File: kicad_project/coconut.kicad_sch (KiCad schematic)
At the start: 77 parts

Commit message: change the layout
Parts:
- K_32: footprint MX_Only:MXOnly-1U-NoLED -> MX_Only:MXOnly-1.25U-NoLED
- K_34: footprint MX_Only:MXOnly-1.5U-NoLED -> MX_Only:MXOnly-1.25U-NoLED
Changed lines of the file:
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@@
       (effects (font (size 1.524 1.524)) hide)
     )
-    (property "Footprint" "MX_Only:MXOnly-1U-NoLED" (id 2) (at 60.96 101.6 0)
+    (property "Footprint" "MX_Only:MXOnly-1.25U-NoLED" (id 2) (at 60.96 101.6 0)
       (effects (font (size 1.524 1.524)) hide)
     )
@@
       (effects (font (size 1.524 1.524)) hide)
     )
-    (property "Footprint" "MX_Only:MXOnly-1.5U-NoLED" (id 2) (at 111.76 101.6 0)
+    (property "Footprint" "MX_Only:MXOnly-1.25U-NoLED" (id 2) (at 111.76 101.6 0)
       (effects (font (size 1.524 1.524)) hide)
     )
@@
     )
     (path "/674840e5-a567-4807-bd27-40d0d1083fb1"
-      (reference "K_32") (unit 1) (value "KEYSW") (footprint "MX_Only:MXOnly-1U-NoLED")
+      (reference "K_32") (unit 1) (value "KEYSW") (footprint "MX_Only:MXOnly-1.25U-NoLED")
     )
     (path "/89cb937e-26ca-48ab-af86-700433b6247b"
@@
     )
     (path "/b670bfa7-a8b0-4c33-afe5-e5a7d5911028"
-      (reference "K_34") (unit 1) (value "KEYSW") (footprint "MX_Only:MXOnly-1.5U-NoLED")
+      (reference "K_34") (unit 1) (value "KEYSW") (footprint "MX_Only:MXOnly-1.25U-NoLED")
     )
     (path "/93a698a0-07b2-4e84-93ac-1d917cde8321"

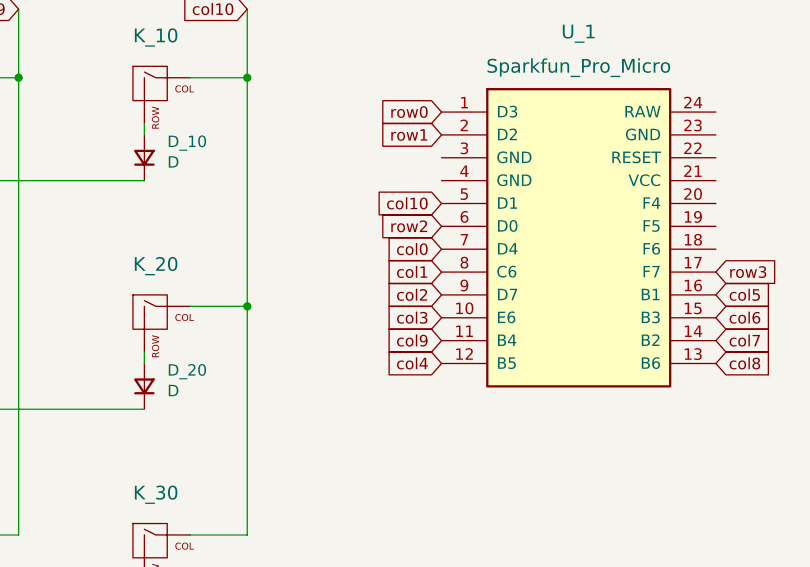
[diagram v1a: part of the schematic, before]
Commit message: fix mismatch
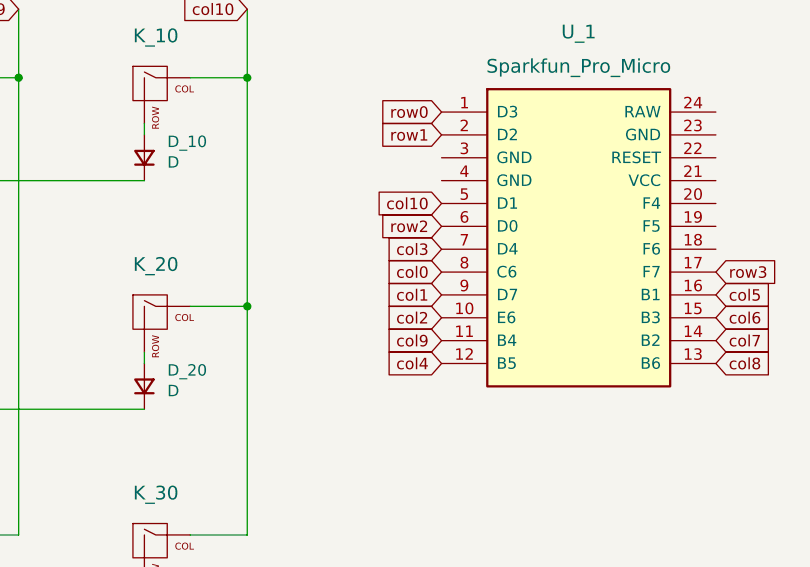
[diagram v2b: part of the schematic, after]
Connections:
- net col0: now also U_1.8 (C6); no longer U_1.7 (D4)
- net col1: now also U_1.9 (D7); no longer U_1.8 (C6)
- net col2: now also U_1.10 (E6); no longer U_1.9 (D7)
- net col3: now also U_1.7 (D4); no longer U_1.10 (E6)
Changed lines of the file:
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@@
     )
   )
-  (global_label "col2" (shape input) (at 321.31 48.26 180) (fields_autoplaced)
+  (global_label "col2" (shape input) (at 321.31 50.8 180) (fields_autoplaced)
     (effects (font (size 1.27 1.27)) (justify right))
-    (property "Intersheet References" "${INTERSHEET_REFS}" (id 0) (at 314.8734 48.1806 0)
+    (property "Intersheet References" "${INTERSHEET_REFS}" (id 0) (at 314.8734 50.7206 0)
       (effects (font (size 1.27 1.27)) (justify right) hide)
     )
@@
     )
   )
-  (global_label "col0" (shape input) (at 321.31 43.18 180) (fields_autoplaced)
+  (global_label "col0" (shape input) (at 321.31 45.72 180) (fields_autoplaced)
     (effects (font (size 1.27 1.27)) (justify right))
-    (property "Intersheet References" "${INTERSHEET_REFS}" (id 0) (at 314.8734 43.1006 0)
+    (property "Intersheet References" "${INTERSHEET_REFS}" (id 0) (at 314.8734 45.6406 0)
       (effects (font (size 1.27 1.27)) (justify right) hide)
     )
@@
     )
   )
-  (global_label "col1" (shape input) (at 321.31 45.72 180) (fields_autoplaced)
+  (global_label "col1" (shape input) (at 321.31 48.26 180) (fields_autoplaced)
     (effects (font (size 1.27 1.27)) (justify right))
-    (property "Intersheet References" "${INTERSHEET_REFS}" (id 0) (at 314.8734 45.6406 0)
+    (property "Intersheet References" "${INTERSHEET_REFS}" (id 0) (at 314.8734 48.1806 0)
       (effects (font (size 1.27 1.27)) (justify right) hide)
     )
@@
     )
   )
-  (global_label "col3" (shape input) (at 321.31 50.8 180) (fields_autoplaced)
+  (global_label "col3" (shape input) (at 321.31 43.18 180) (fields_autoplaced)
     (effects (font (size 1.27 1.27)) (justify right))
-    (property "Intersheet References" "${INTERSHEET_REFS}" (id 0) (at 314.8734 50.7206 0)
+    (property "Intersheet References" "${INTERSHEET_REFS}" (id 0) (at 314.8734 43.1006 0)
       (effects (font (size 1.27 1.27)) (justify right) hide)
     )
